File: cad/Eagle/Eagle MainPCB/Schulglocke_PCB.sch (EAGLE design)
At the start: 34 parts, among them IC1 SFH6156, IC2 SFH6156, K1 JS-M1-9V-5, M1 DS3231SHIELD, M2 EMC28J60SHIELD, M3 WAVESHAREDISPLAY, Q1 BSS123, Q2 BSS123

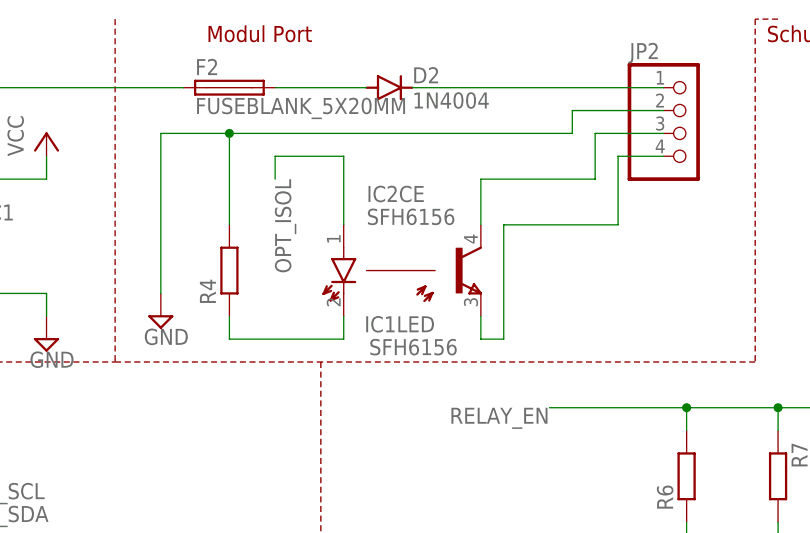
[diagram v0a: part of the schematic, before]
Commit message: before change
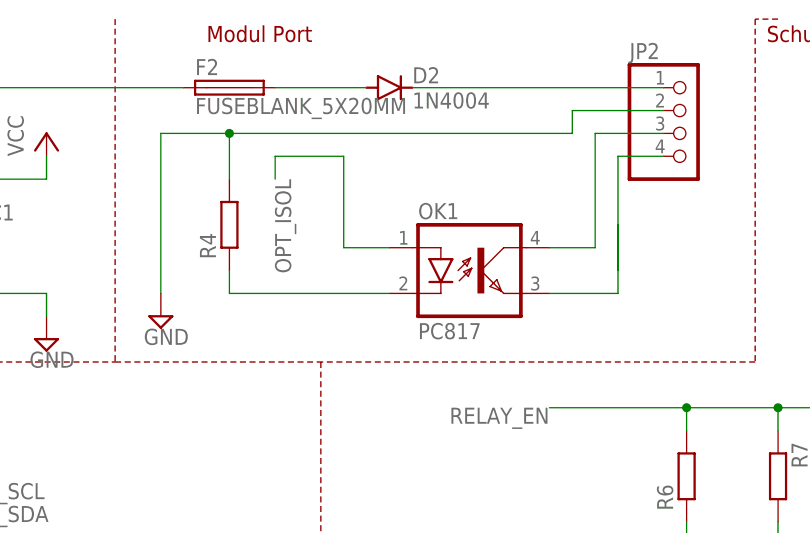
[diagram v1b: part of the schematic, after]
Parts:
- removed IC1, IC2: SFH6156, optocoupler:SFH6156
- added OK1: PC817, optocoupler:PC817
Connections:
- net N$19: now also OK1.C; no longer IC1LED.K
- net N$6: now also OK1.COL; no longer IC2CE.C
- net N$7: now also OK1.EMIT; no longer IC2CE.E
- net OPT_ISOL: now also OK1.A; no longer IC1LED.A
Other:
- moved on the sheet: R4

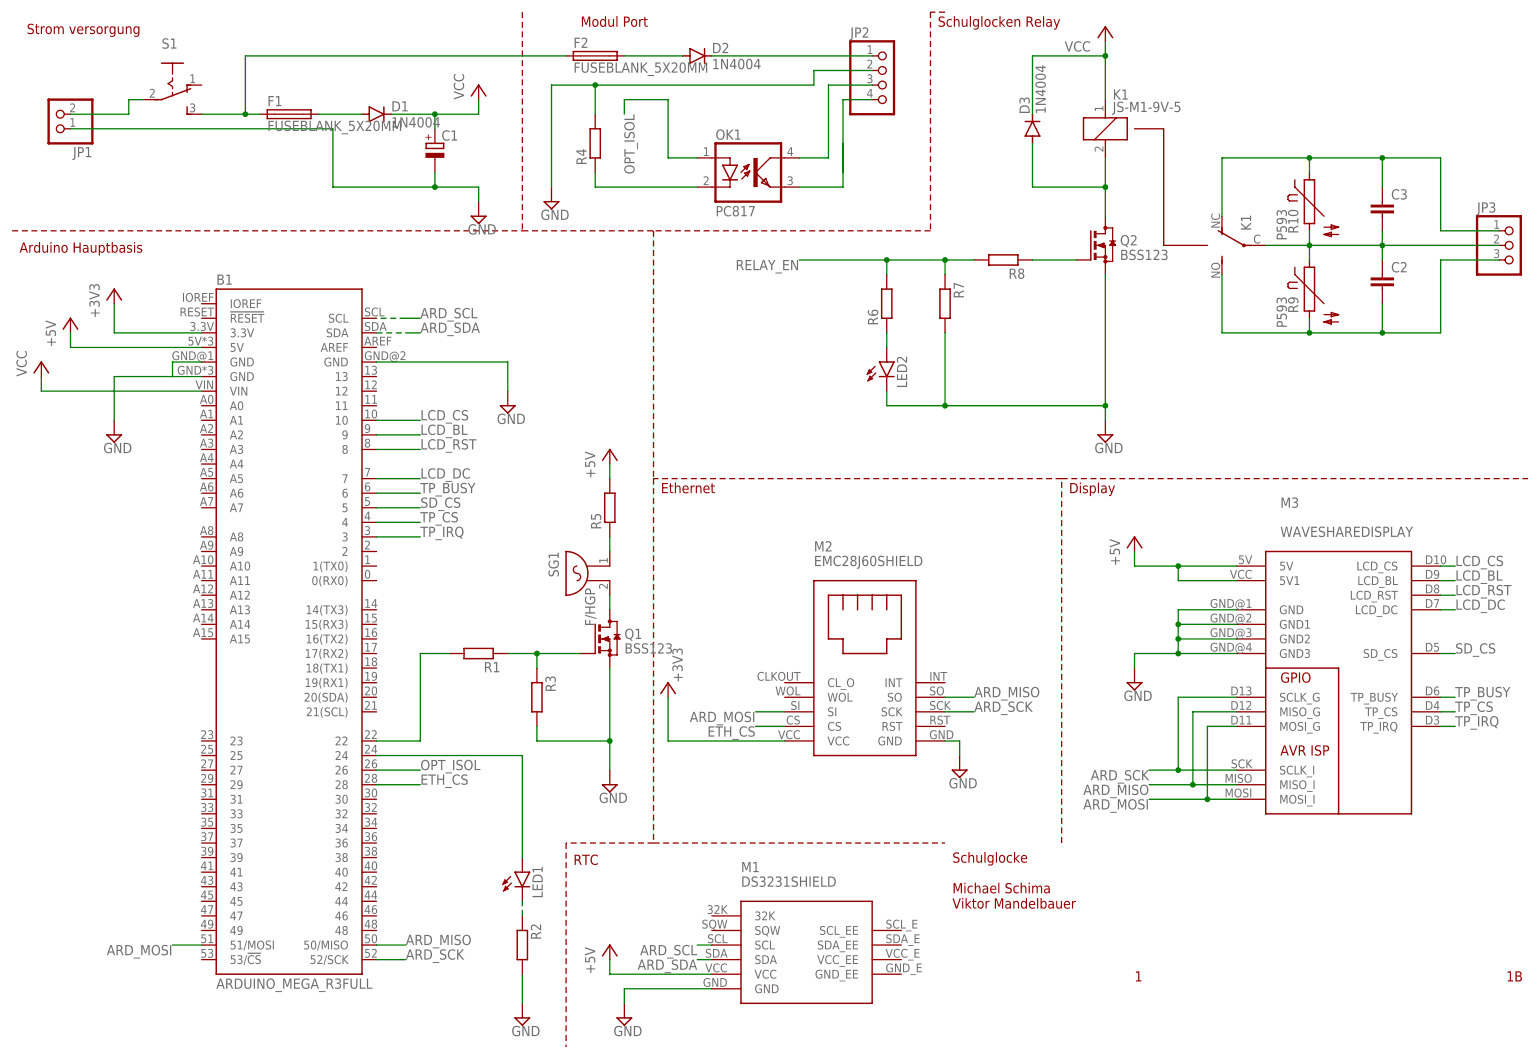
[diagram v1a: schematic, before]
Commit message: leiterplatte plaziert
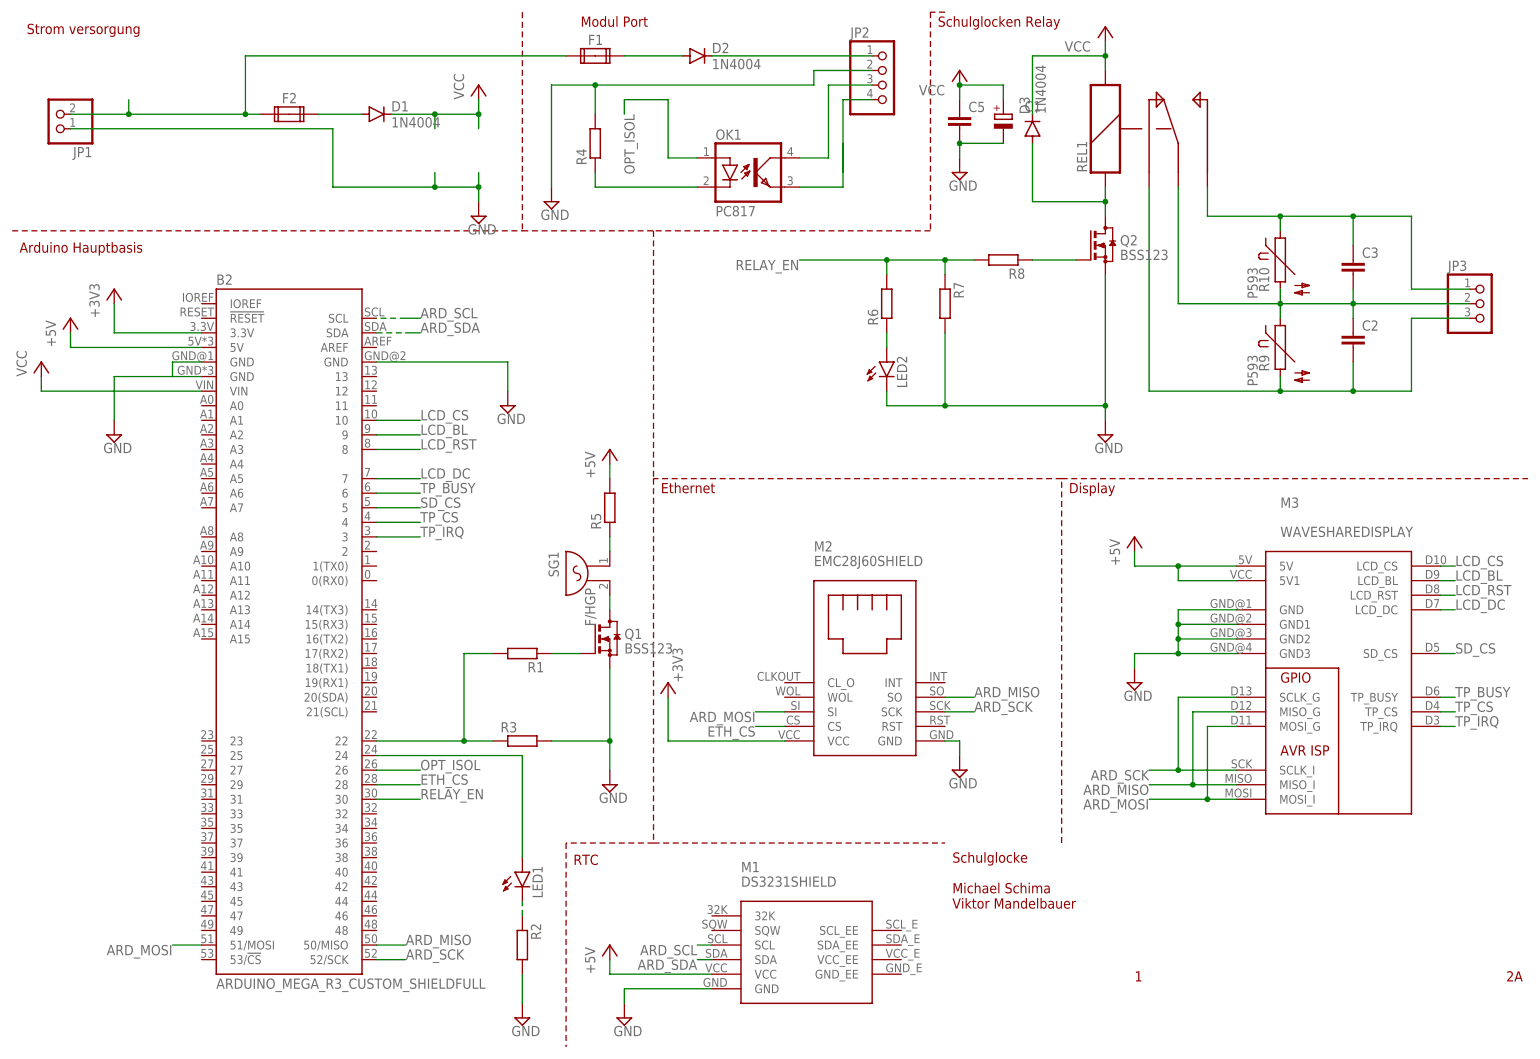
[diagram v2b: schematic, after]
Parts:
- removed B1: ARDUINO_MEGA_R3FULL, sparkfun eagle:ARDUINO_MEGA_R3FULL
- removed K1: JS-M1-9V-5, relay:JS-M1-9V-5
- removed S1: (no value), switch:255SB
- added B2: ARDUINO_MEGA_R3_CUSTOM_SHIELDFULL, customlib:ARDUINO_MEGA_R3_CUSTOM_SHIELDFULL
- added C5: (no value), rcl:C-EUC1206K
- added REL1: (no value), special:REL-5PIN
- F1, F2: value FUSEBLANK_5X20MM -> (none); device fuse:FUSEBLANK_5X20MM -> special:FUSE2P
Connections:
- removed net N$11: JP1.2, S1.P
- new net N$18: B2.30
- net +3V3: now also B2.3.3V; no longer B1.3.3V
- net +5V: now also B2.5V; no longer B1.5V
- net ARD_MISO: now also B2.50/MISO; no longer B1.50/MISO
- net ARD_MOSI: now also B2.51/MOSI; no longer B1.51/MOSI
- net ARD_SCK: now also B2.52/SCK; no longer B1.52/SCK
- net ARD_SCL: now also B2.SCL; no longer B1.SCL
- net ARD_SDA: now also B2.SDA; no longer B1.SDA
- net ETH_CS: now also B2.28; no longer B1.28
- net GND: now also B2.GND, B2.GND@2, B2.GND@3, C5.2; no longer B1.GND, B1.GND@2, B1.GND@3
- net LCD_BL: now also B2.9; no longer B1.9
- net LCD_CS: now also B2.10; no longer B1.10
- net LCD_DC: now also B2.7; no longer B1.7
- net LCD_RST: now also B2.8; no longer B1.8
- net N$1: now also REL1.C; no longer K12.P
- net N$10: now also REL1.S1; no longer K11.2
- net N$12: now also B2.24; no longer B1.24
- net N$16: now also B2.22, R3.1; no longer B1.22
- net N$17: no longer R3.1
- net N$2: now also REL1.O; no longer K12.O
- net N$3: now also REL1.S; no longer K12.S
- net N$4: now also F1.2A; no longer F2.2
- net N$8: now also F1.1A, F2.1A, JP1.2; no longer F1.1, F2.1, S1.S
- net N$9: now also F2.2A; no longer F1.2
- net OPT_ISOL: now also B2.26; no longer B1.26
- net SD_CS: now also B2.5; no longer B1.5
- net TP_BUSY: now also B2.6; no longer B1.6
- net TP_CS: now also B2.4; no longer B1.4
- net TP_IRQ: now also B2.3; no longer B1.3
- net VCC: now also B2.VIN, C5.1, REL1.S2; no longer B1.VIN, K11.1
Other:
- note added: "2A"
- note removed: "1B"
- moved on the sheet: C1, C2, C3, JP3, R1, R10, R3, R9
